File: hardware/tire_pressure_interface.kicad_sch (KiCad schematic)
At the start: 1 part, among them U3 XIAO-ESP32-S3-DIP

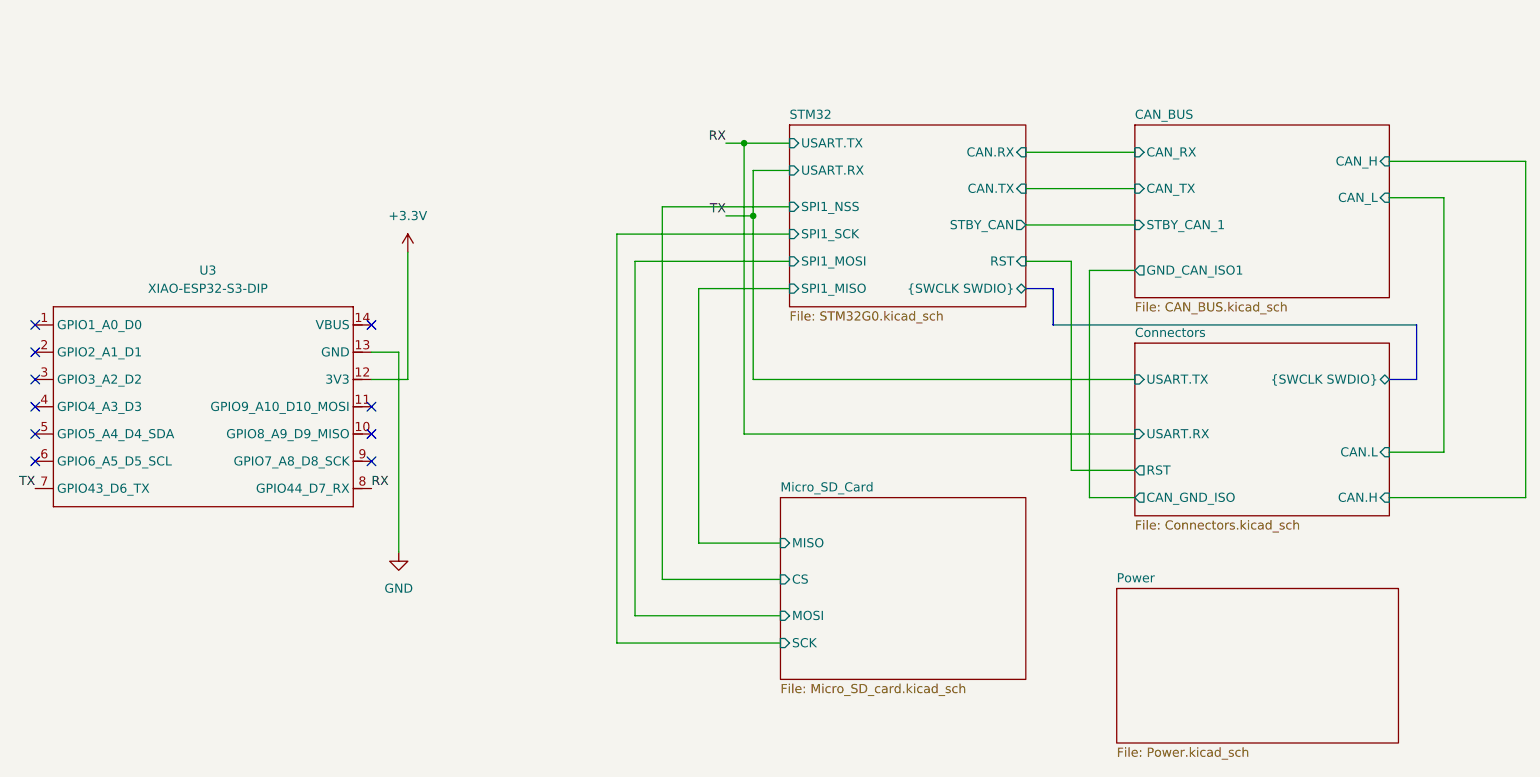
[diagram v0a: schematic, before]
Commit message: reorganization of project folders acording to templates
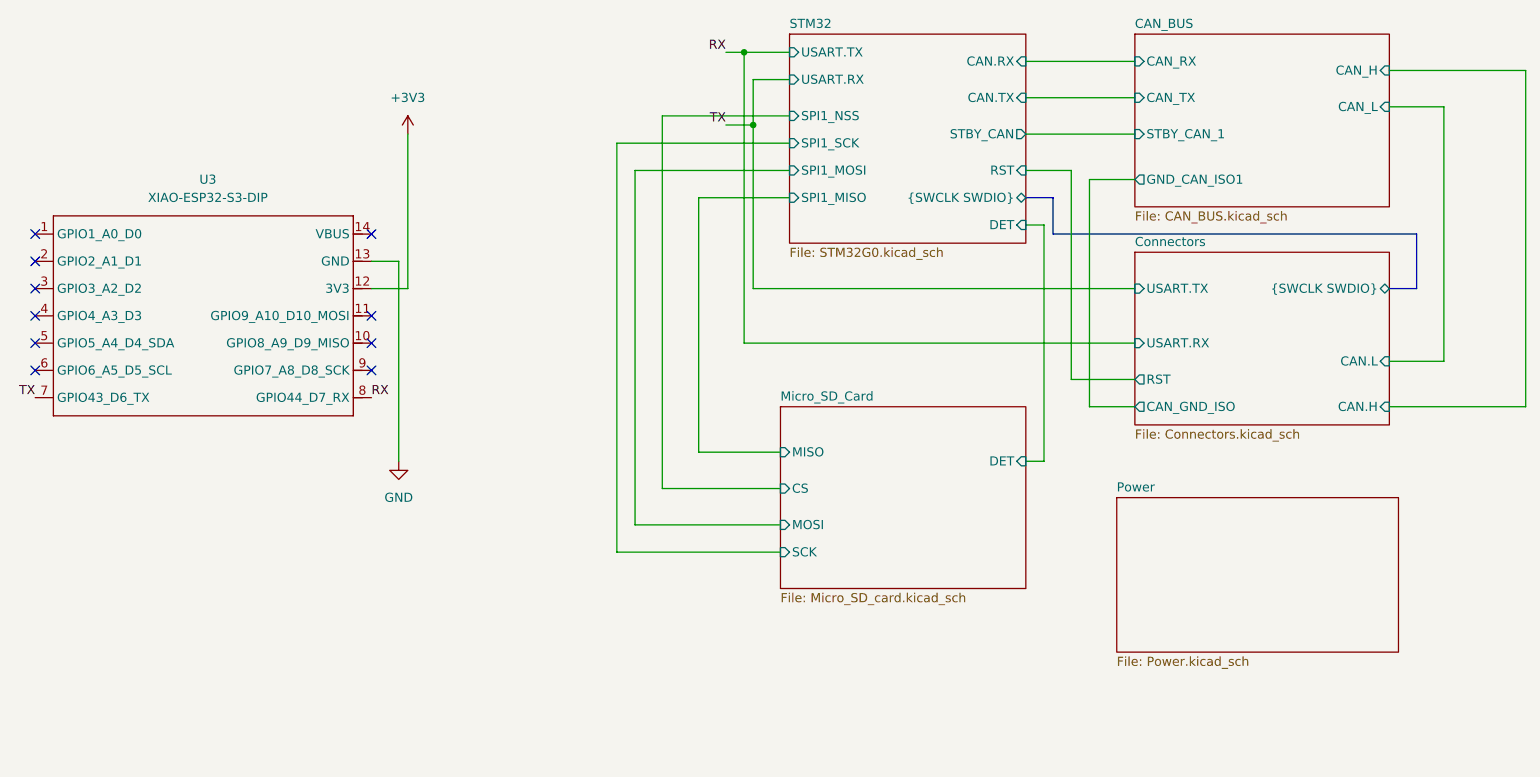
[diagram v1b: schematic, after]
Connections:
- net +3.3V renamed +3V3
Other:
- sheet Micro_SD_Card ports: added DET; removed none
- sheet STM32 ports: added DET; removed none
- company: (none) -> Author:
